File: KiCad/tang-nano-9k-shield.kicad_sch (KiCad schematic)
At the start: 97 parts, among them J1 Barrel_Jack, J2 AudioJack3, J3 USB_C_Receptacle_USB2.0_16P, J4 I2C_headers, J5 DE15_Socket_HighDensity_Mount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, J6 DE9_Socket_MountingHoles, J7 SPI_headers, Q1 SS8050, SW1 RotaryEncoder_Switch_MP, SW2 SW_Push, SW3 SW_Push, SW4 SW_Push, U1 Tang Nano 9K, U10 MAX3232, U3 TPS563201DDCR, U4 AMS1117-3.3, U5 PT8211, U6 TPA6132A2RTE, U7 USBLC6-2SC6, U8 RP2040, U9 W25Q32JVZP, Y1 X322512MSB4SI

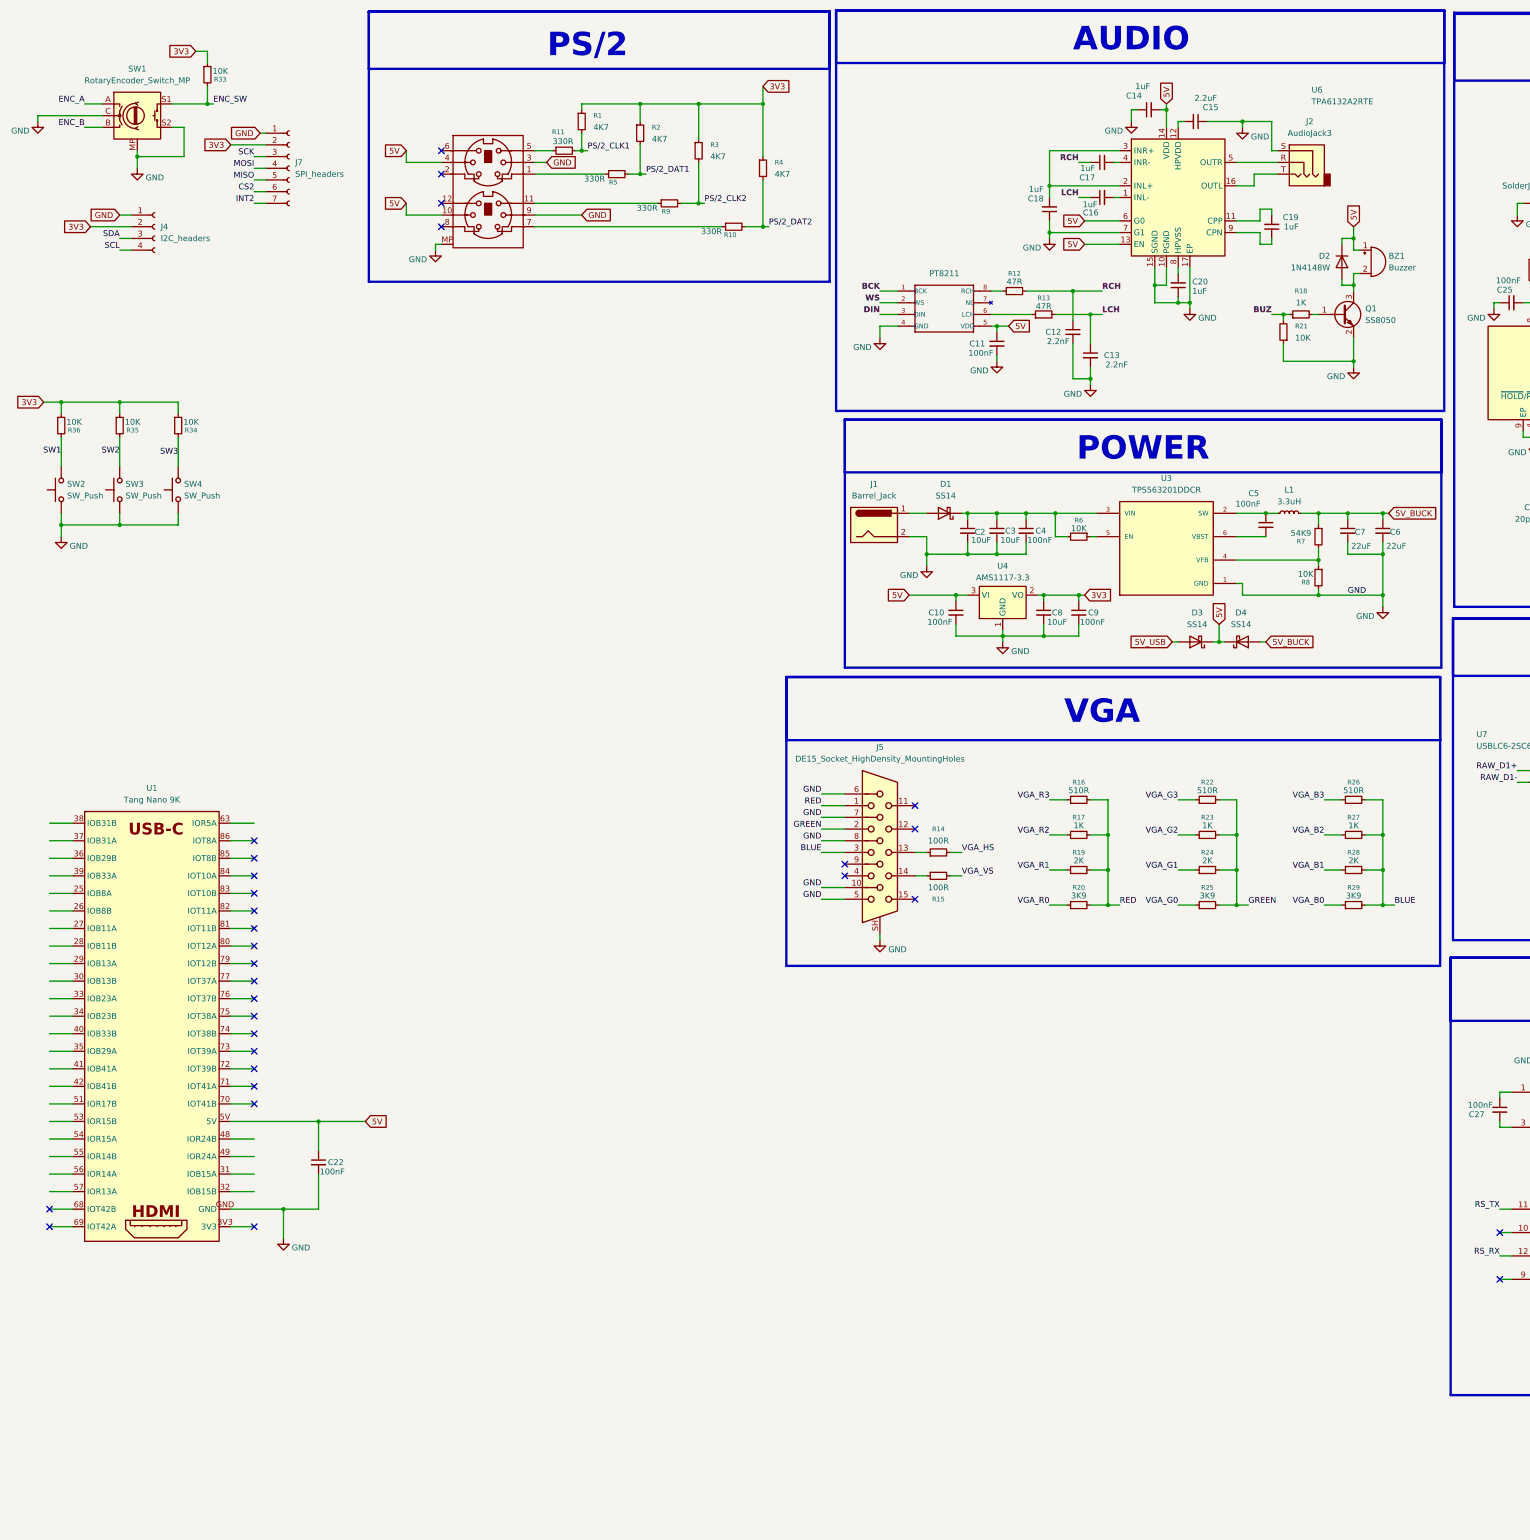
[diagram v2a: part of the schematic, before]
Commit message: Add files via upload
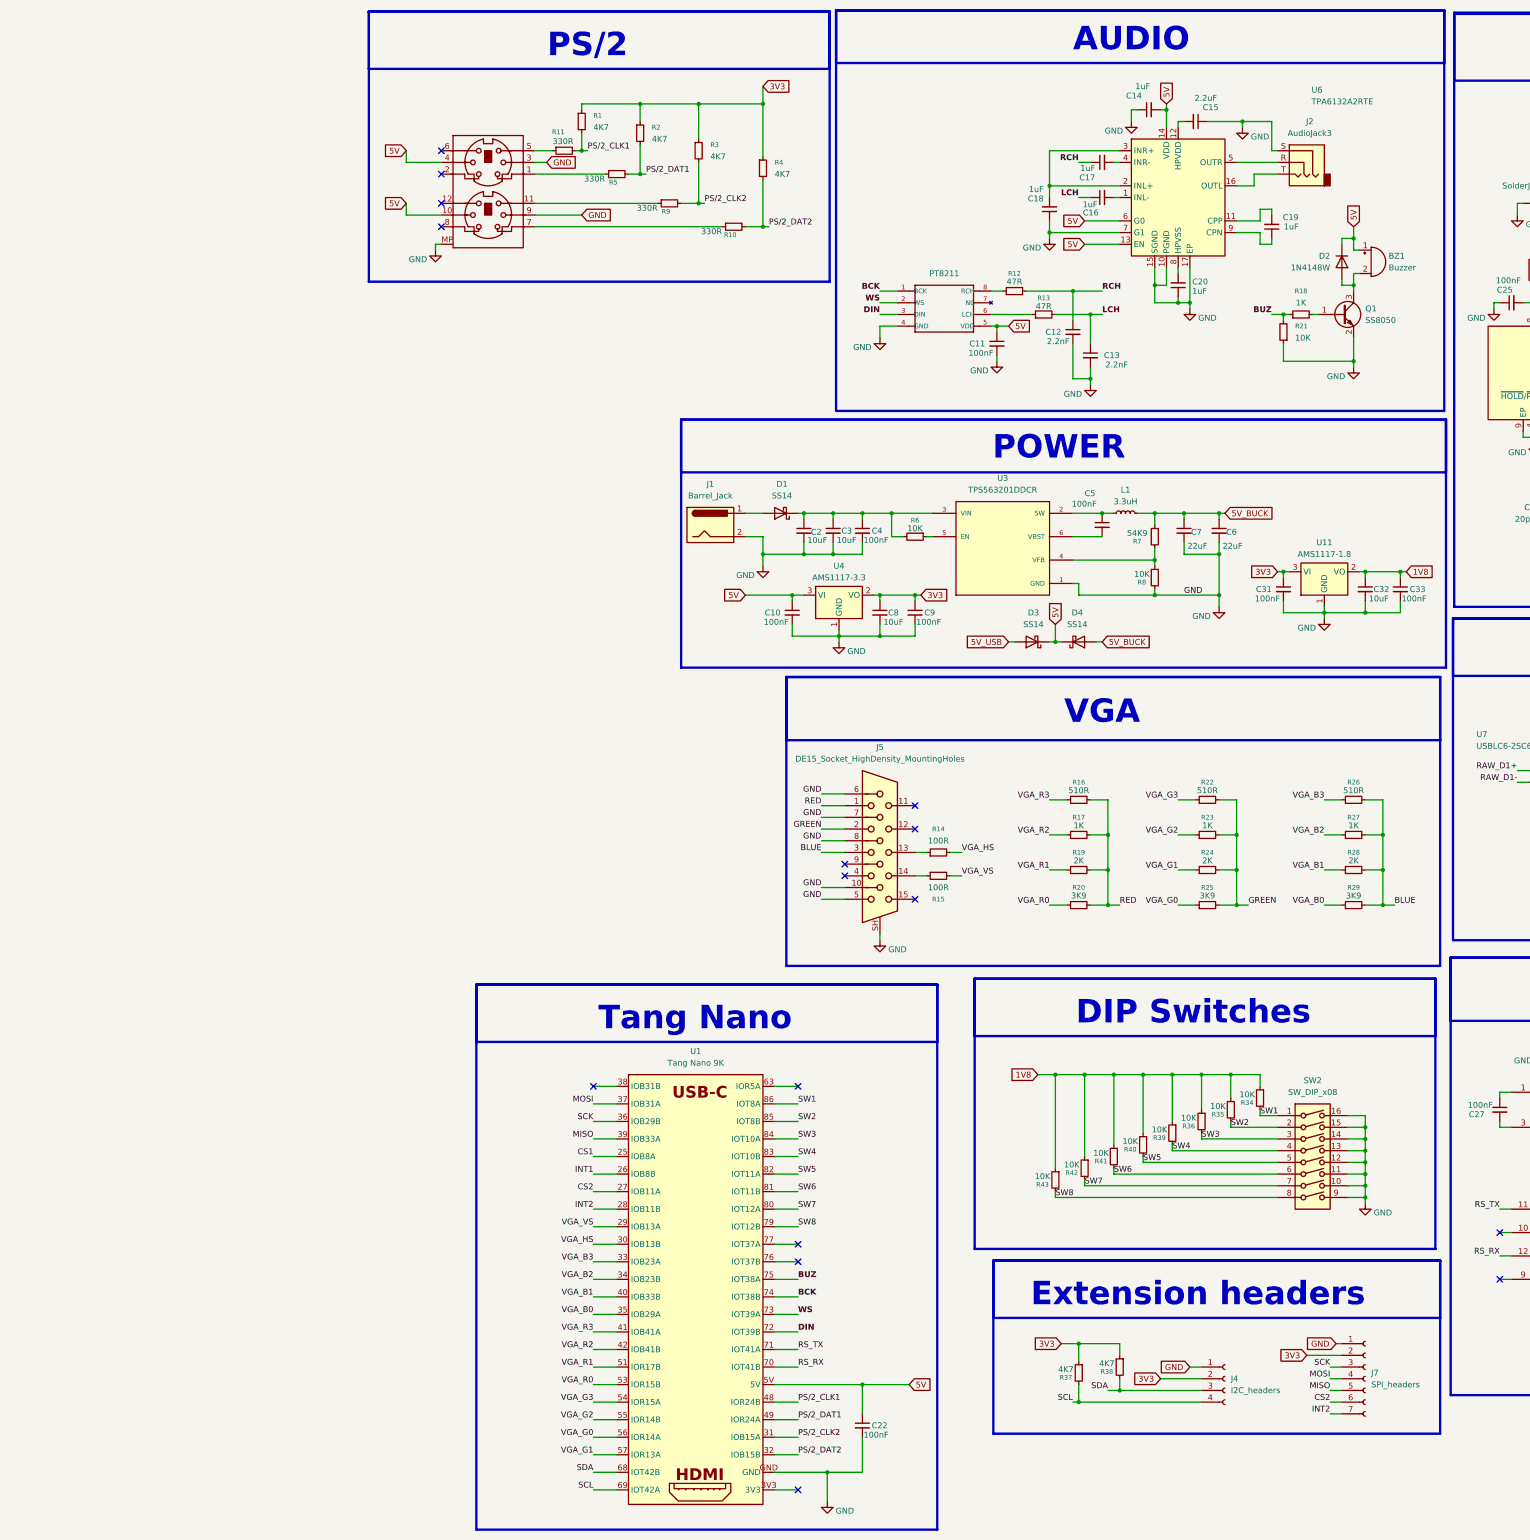
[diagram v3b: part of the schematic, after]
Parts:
- removed R33: 10K, symbol Device:R_Small
- removed SW1: RotaryEncoder_Switch_MP, symbol Device:RotaryEncoder_Switch_MP
- removed SW2, SW3, SW4: SW_Push, symbol Switch:SW_Push
- added C31, C33: 100nF, symbol Device:C_Small
- added C32: 10uF, symbol Device:C_Small
- added R37, R38: 4K7, symbol Device:R_Small
- added R39, R40, R41, R42, R43: 10K, symbol Device:R_Small
- added SW2: SW_DIP_x08, symbol Switch:SW_DIP_x08
- added U11: AMS1117-1.8, Package_TO_SOT_SMD:SOT-223-3_TabPin2, symbol Regulator_Linear:AMS1117-1.8
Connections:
- net 3V3: now also C31.1, R37.1, R38.1, U11.3 (VI); no longer R34.1, R35.1, R36.1
- net BCK: now also U1.74 (IOT38B)
- net BUZ: now also U1.75 (IOT38A)
- net CS1: now also U1.25 (IOB8A)
- net CS2: now also U1.27 (IOB11A)
- net DIN: now also U1.72 (IOT39B)
- net GND: now also C31.2, C32.2, C33.2, SW2.10, SW2.11, SW2.12, SW2.13, SW2.14, SW2.15, SW2.16, SW2.9, U11.1 (GND)
- net INT1: now also U1.26 (IOB8B)
- net INT2: now also U1.28 (IOB11B)
- net MISO: now also U1.39 (IOB33A)
- net MOSI: now also U1.37 (IOB31A)
- net PS/2_CLK1: now also U1.48 (IOR24B)
- net PS/2_CLK2: now also U1.31 (IOB15A)
- net PS/2_DAT1: now also U1.49 (IOR24A)
- net PS/2_DAT2: now also U1.32 (IOB15B)
- net RS_RX: now also U1.70 (IOT41B)
- net RS_TX: now also U1.71 (IOT41A)
- net SCK: now also U1.36 (IOB29B)
- net SCL: now also U1.69 (IOT42A), R37.2
- net SDA: now also U1.68 (IOT42B), R38.2
- net SW1: now also R34.2, U1.86 (IOT8A), SW2.1; no longer R36.2
- net SW2: now also U1.85 (IOT8B), SW2.2
- net SW3: now also R36.2, U1.84 (IOT10A), SW2.3; no longer R34.2
- net VGA_B0: now also U1.35 (IOB29A)
- net VGA_B1: now also U1.40 (IOB33B)
- net VGA_B2: now also U1.34 (IOB23B)
- net VGA_B3: now also U1.33 (IOB23A)
- net VGA_G0: now also U1.56 (IOR14A)
- net VGA_G1: now also U1.57 (IOR13A)
- net VGA_G2: now also U1.55 (IOR14B)
- net VGA_G3: now also U1.54 (IOR15A)
- net VGA_HS: now also U1.30 (IOB13B)
- net VGA_R0: now also U1.53 (IOR15B)
- net VGA_R1: now also U1.51 (IOR17B)
- net VGA_R2: now also U1.42 (IOB41B)
- net VGA_R3: now also U1.41 (IOB41A)
- net VGA_VS: now also U1.29 (IOB13A)
- net WS: now also U1.73 (IOT39A)
- net SW8: now reaches U1.79 (IOT12B)
- net SW8: now also R43.2, SW2.8
- net SW7: now reaches U1.80 (IOT12A)
- net SW7: now also R42.2, SW2.7
- net SW6: now reaches U1.81 (IOT11B)
- net SW6: now also R41.2, SW2.6
- net SW5: now reaches U1.82 (IOT11A)
- net SW5: now also R40.2, SW2.5
- net SW4: now reaches U1.83 (IOT10B)
- net SW4: now also R39.2, SW2.4
- new net 1V8: C32.1, C33.1, R34.1, R35.1, R36.1, R39.1, R40.1, R41.1, R42.1, R43.1, U11.2 (VO)
- no-connect marks 68 -> 54
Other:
- note added: "DIP Switches"
- note added: "Extension headers"
- note added: "Tang Nano"
- moved on the sheet: C10, C2, C22, C3, C4, C5, C6, C7, C8, C9, D1, D3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
